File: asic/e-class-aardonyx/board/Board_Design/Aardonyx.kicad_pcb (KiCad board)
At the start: 4 copper layers, 306 parts, among them J1 USB_B_6PIN, J10 Conn_1x6_F, J11 Conn_1x6_F, J12 Conn_1x3_M, J13 Conn_1x8_F, J14 Conn_1x6_F, J15 Conn_1x10, J16 Conn_1x8_F, J17 USB_OTG, J18 Conn_1x3_M, J19 Conn_1x3_M, J2 Conn_1x8, J3 Conn_1x3_M, J4 Conn_1x4, J5 PJ-202H PWRJACK, J6 Conn_1x3_M, J7 Conn_1x4, J8 Conn_1x3_M, J9 Conn_1x8, Q1 FDN339AN, SW1 SW_SPST, SW2 FSM2JSMAATR, SW3 SW_DIP_x03, U1 FT2232H, U10 TPS7A7002DDAR, U11 ADM1085, U12 ADM1085, U13 TPS7A7002DDAR, U14 74AUP1G09GW, U15 SKT32E, U16 93LC56BT-I_OT, U2 IS42S32160F-TSOP2, U3 CDCE913PW, U4 TPS54627DDAR, U5 CAT24M01WI-GT3, U6 IS25LP256x-xM, U7 ADC128S102CIMTX/NOPB, U8 LSF0108PWR, U9 LSF0108PWR, Y1 12MHz, Y2 27MHz

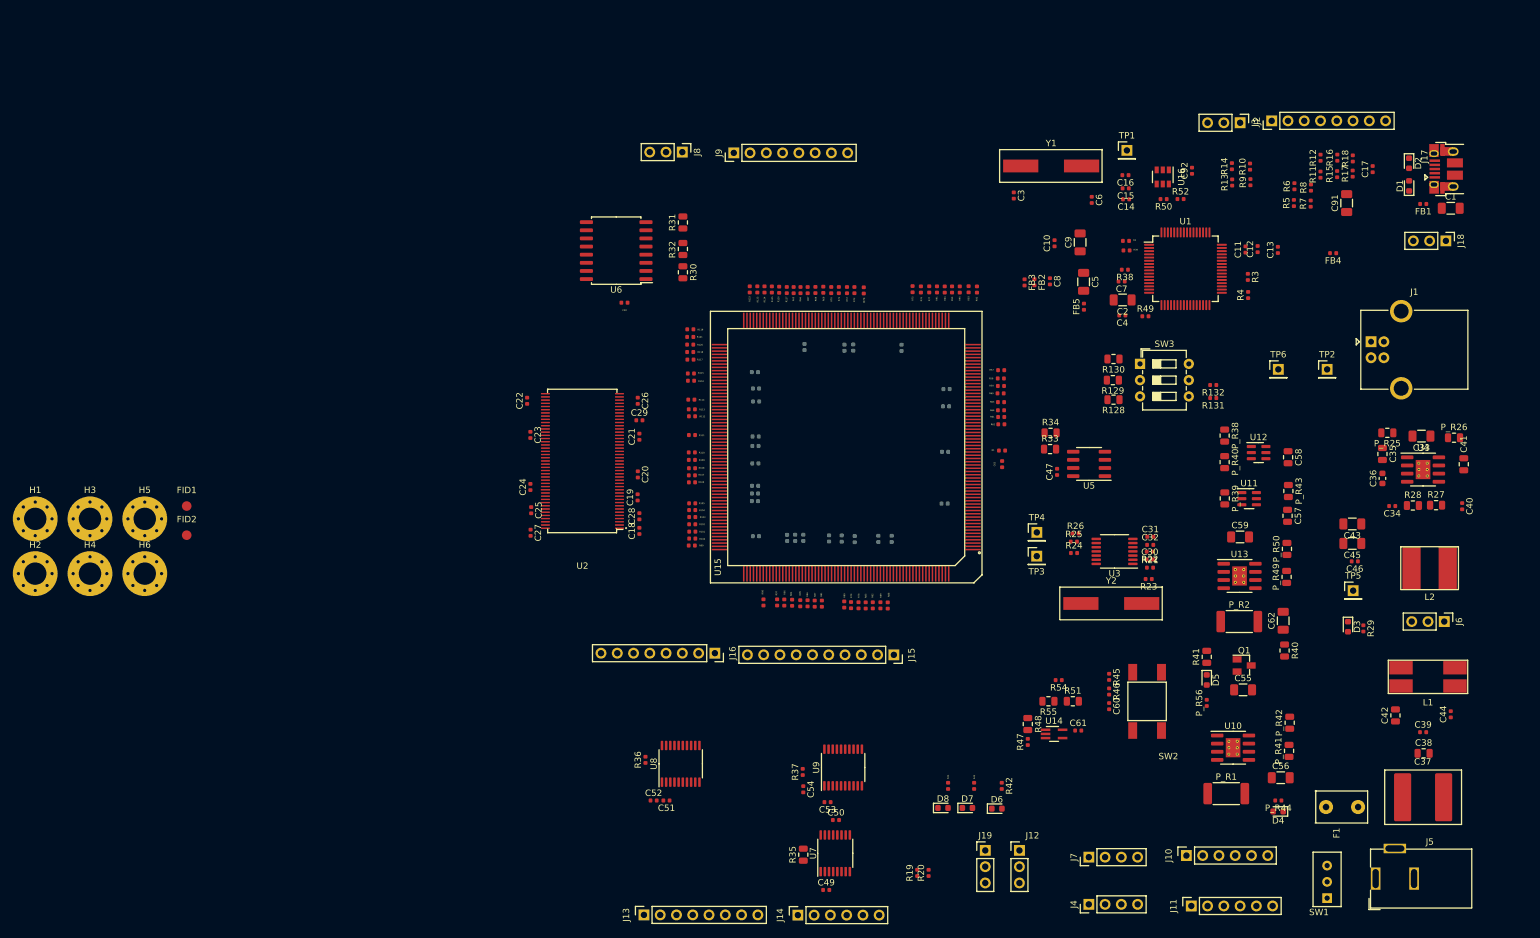
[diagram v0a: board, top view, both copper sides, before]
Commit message: updated the component
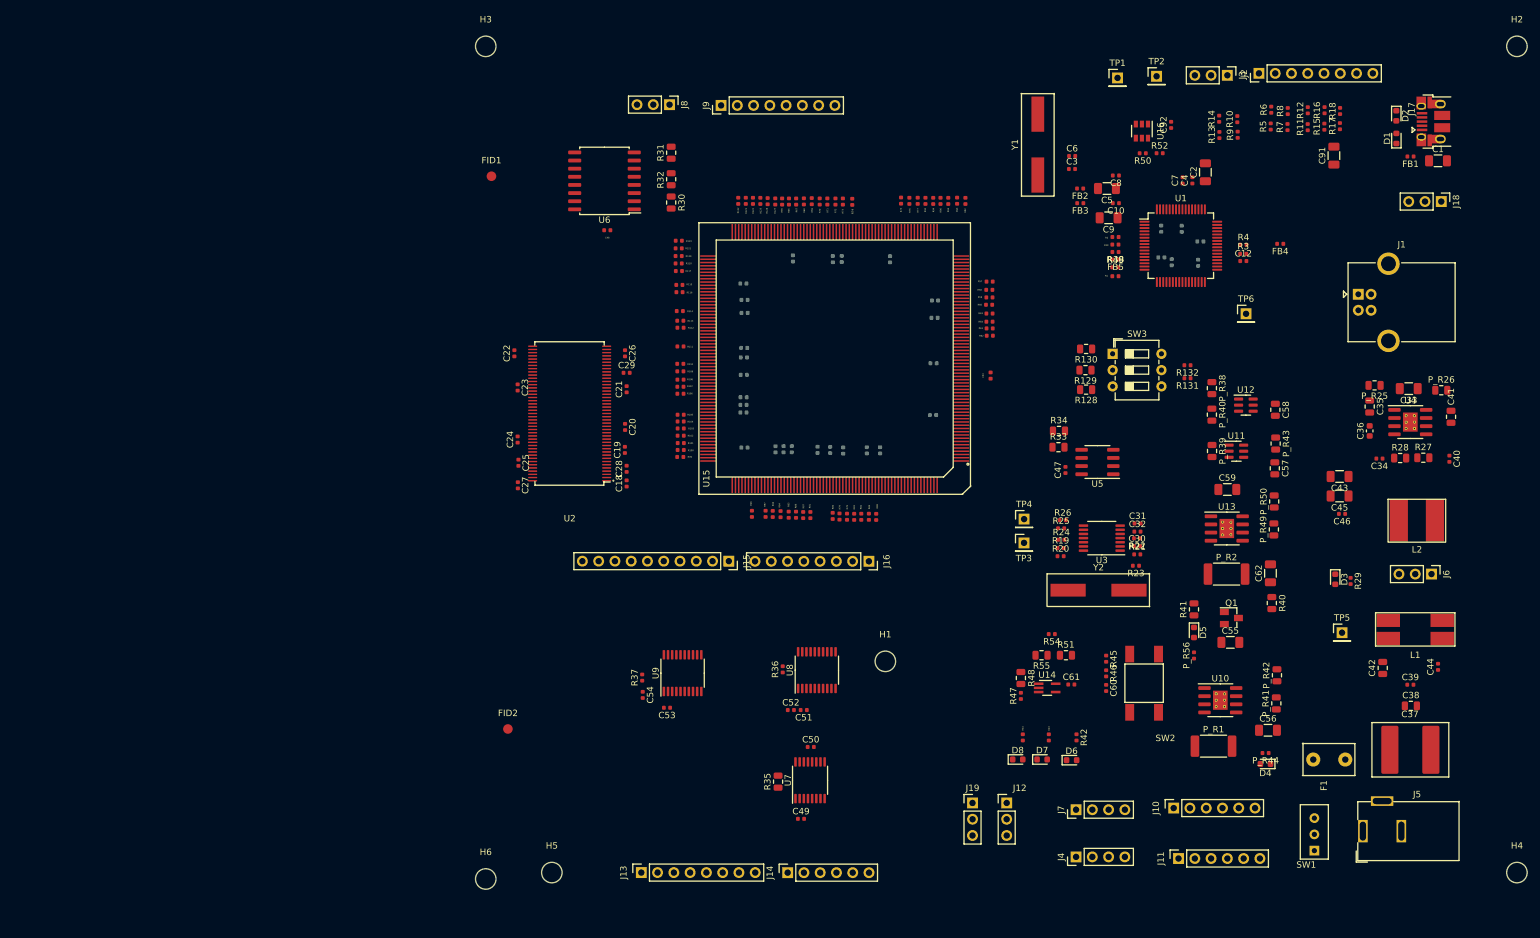
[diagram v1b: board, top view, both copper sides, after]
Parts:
- C11, C13, C14, C15, C16, C17: moved to B.Cu
- H1, H2, H3, H4, H5, H6: footprint MountingHole:MountingHole_3.5mm_Pad_Via -> MountingHole:MountingHole_3.2mm_M3
- moved H2 245.6 mm to (275.0, 25.0)
- moved H4 227.6 mm to (275.0, 154.0)
- moved H1 134.6 mm to (176.4, 121.0)
- moved H3 96.2 mm to (114.0, 25.0)
- moved H5 84.2 mm to (124.3, 154.0)
- moved H6 71.5 mm to (114.0, 155.0)
- moved FID1 70.1 mm to (114.9, 45.3)
- moved FID2 58.6 mm to (117.5, 131.6)
- moved R19 55.4 mm to (203.8, 103.3), turned to 0 degrees
- moved R20 53.6 mm to (203.8, 104.6), turned to 0 degrees
- moved TP2 52.9 mm to (218.7, 29.7)
- moved R1 32.5 mm to (212.3, 60.9)
- moved C17 31.2 mm to (222.7, 53.5), turned to 270 degrees
- moved J15 29.6 mm to (151.9, 105.4)
- moved C53 29.1 mm to (142.3, 128.3)
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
